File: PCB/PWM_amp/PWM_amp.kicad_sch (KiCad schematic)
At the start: 38 parts, among them J1 Conn_01x06_Pin, J10 XT30UPB-M, J2 Conn_01x06_Pin, J3 Conn_01x02_Pin, J4 Conn_01x02_Pin, J49 XT60PW-M, J5 XT30UPB-M, Q1 FDD8447L, Q2 FDD8447L, U1 VNH5019A-E, U2 VNH5019A-E, U3 NC7SVU04P5X, U4 NC7SVU04P5X

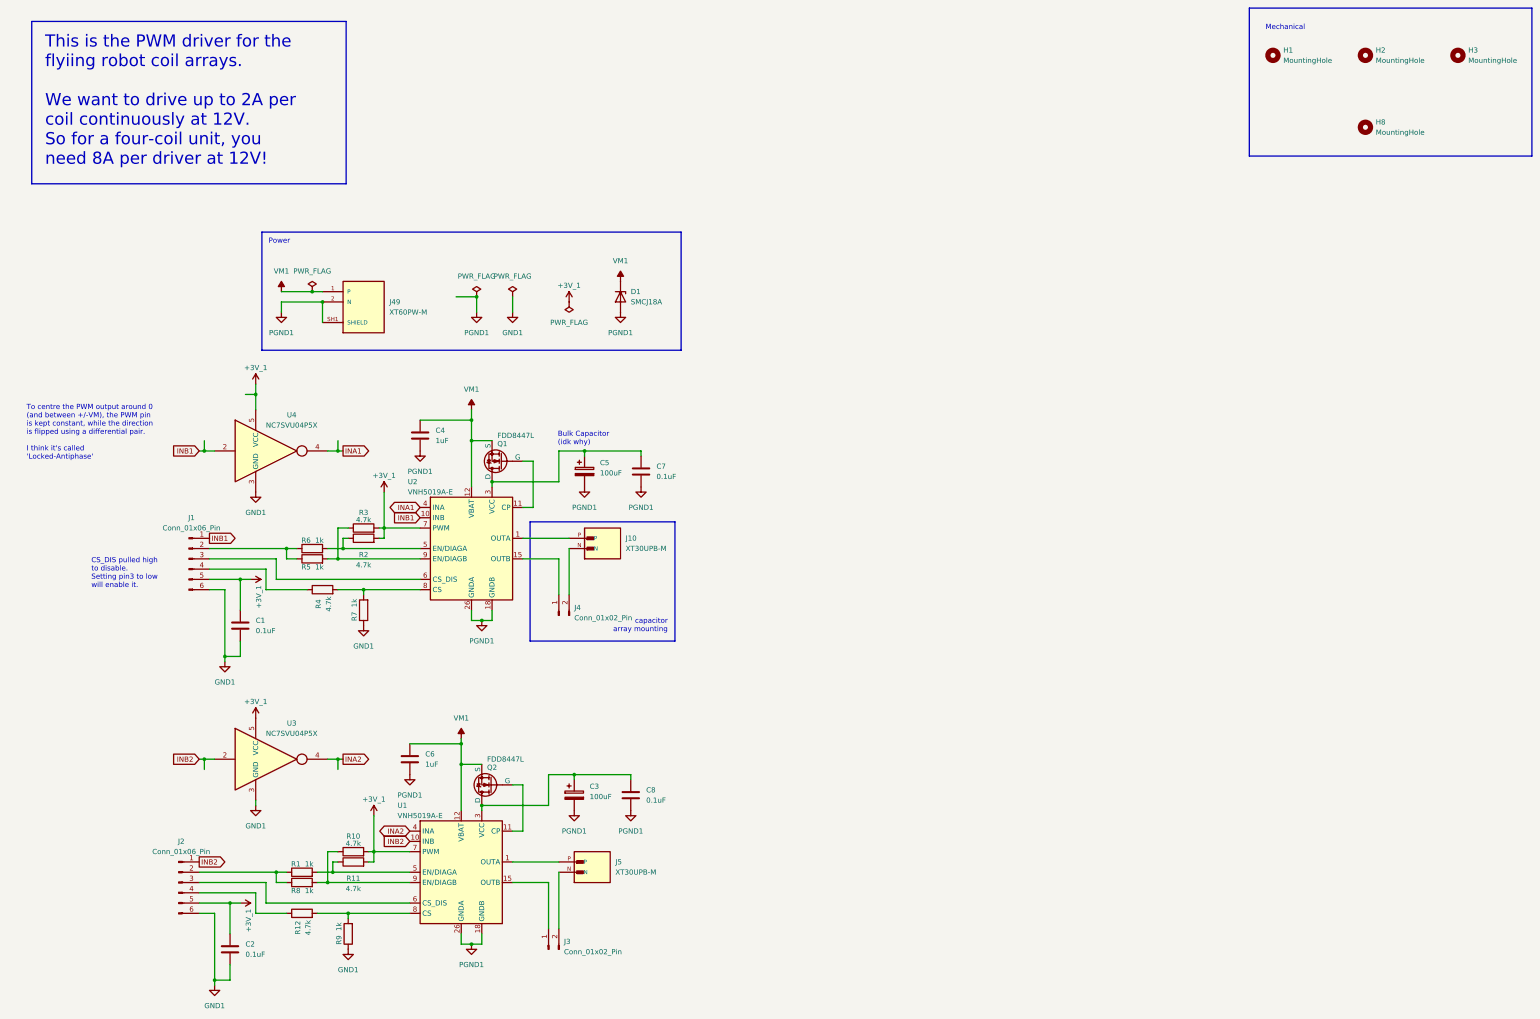
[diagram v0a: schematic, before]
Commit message: added circuits
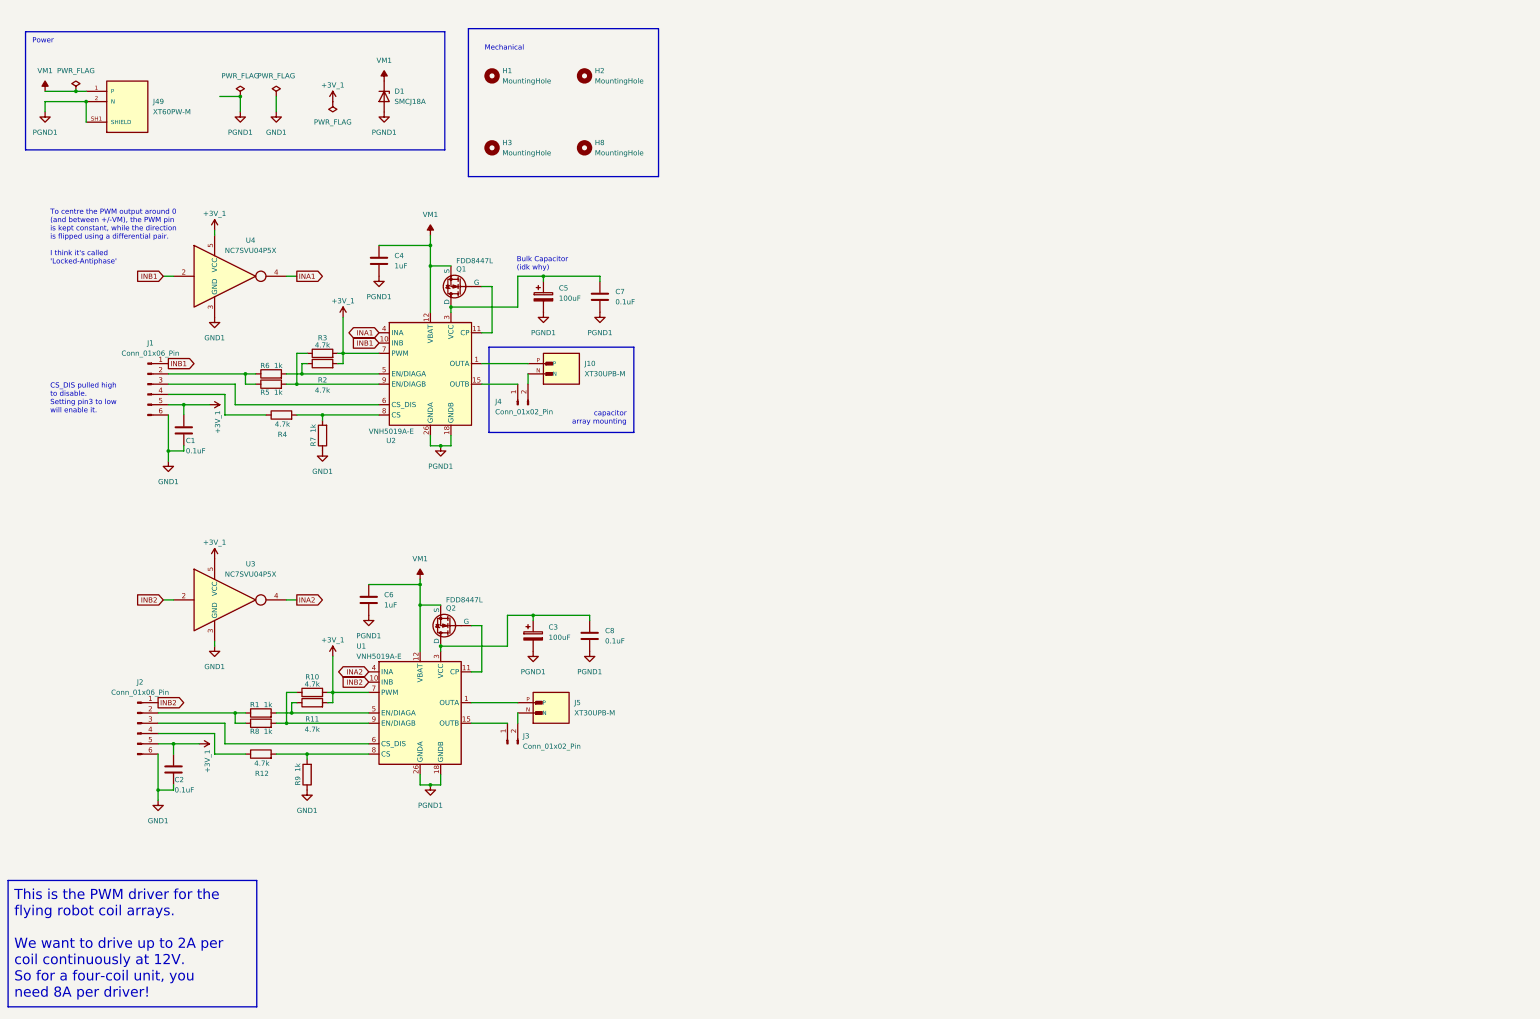
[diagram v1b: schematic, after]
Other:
- note added: "This is the PWM driver for the flying robot coil arrays. We want to drive up to 2A per coil continuously at 12V. So for a four-coil unit, you need 8A per driver!"
- note removed: "This is the PWM driver for the flyiing robot coil arrays. We want to drive up to 2A per coil continuously at 12V. So for a four-coil unit, you need 8A per driver at 12V!"
- company: Kevin Ying - Lin Lab -> Micro Flying Robots - Liwei Lin Lab
- moved on the sheet: C1, C2, C3, C4, C5, C6, C7, C8, D1, H1, H2, H3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
